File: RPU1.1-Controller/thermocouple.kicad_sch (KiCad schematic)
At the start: 5 parts, among them U13 AD8495

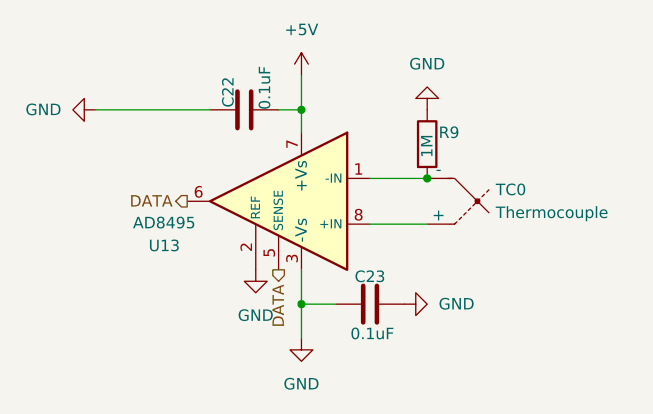
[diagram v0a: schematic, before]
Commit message: A bunch of KiCad Projects
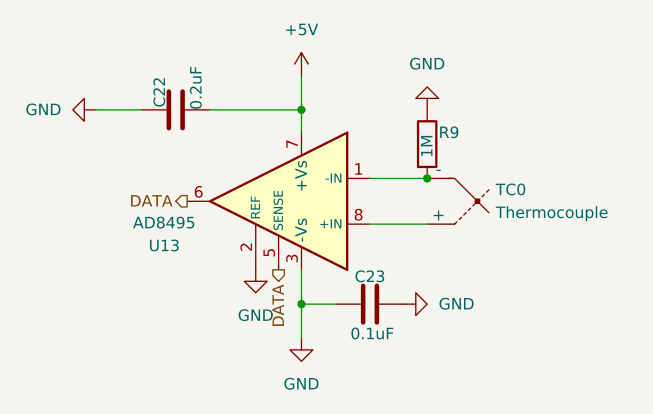
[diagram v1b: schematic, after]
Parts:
- C22: value 0.1uF -> 0.2uF
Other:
- moved on the sheet: C22
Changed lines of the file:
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@@
 	(wire
 		(pts
-			(xy 114.3 68.58) (xy 111.76 68.58)
+			(xy 114.3 68.58) (xy 104.14 68.58)
 		)
 		(stroke
@@
 	(wire
 		(pts
-			(xy 91.44 68.58) (xy 104.14 68.58)
+			(xy 91.44 68.58) (xy 96.52 68.58)
 		)
 		(stroke
@@
 	(symbol
 		(lib_id "Device:C")
-		(at 107.95 68.58 90)
+		(at 100.33 68.58 90)
 		(unit 1)
 		(exclude_from_sim no)
@@
 		(dnp no)
 		(property "Reference" "C22"
-			(at 106.172 68.326 0)
+			(at 98.552 68.326 0)
 			(effects
 				(font
@@
 			)
 		)
-		(property "Value" "0.1uF"
-			(at 110.236 68.58 0)
+		(property "Value" "0.2uF"
+			(at 102.616 68.58 0)
 			(effects
 				(font
@@
 		)
 		(property "Footprint" "Capacitor_SMD:C_0603_1608Metric_Pad1.08x0.95mm_HandSolder"
-			(at 111.76 67.6148 0)
+			(at 104.14 67.6148 0)
 			(effects
 				(font
@@
 		)
 		(property "Datasheet" "~"
-			(at 107.95 68.58 0)
+			(at 100.33 68.58 0)
 			(effects
 				(font
@@
 		)
 		(property "Description" "Unpolarized capacitor"
-			(at 107.95 68.58 0)
-			(effects
-				(font
+			(at 100.33 68.58 0)
+			(effects
+				(font
